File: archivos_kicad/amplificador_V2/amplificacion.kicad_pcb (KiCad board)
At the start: 2 copper layers, 62 x 85.8 mm, 24 parts, among them J1 INPUT_L, J2 OUTPUT_L, J3 ALIMENTACION REJILLA, J4 ALIMENTACION FILAMENTO, J5 INPUT_R, J6 OUTPUT_R

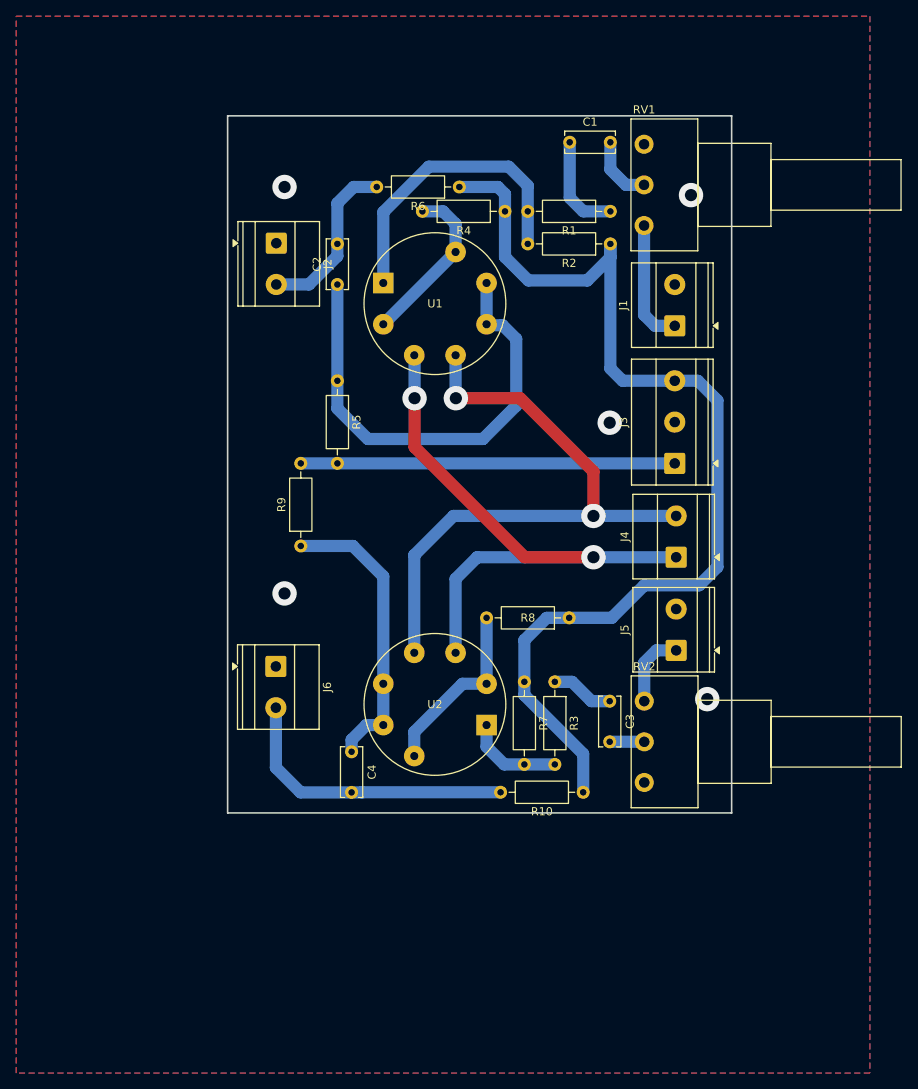
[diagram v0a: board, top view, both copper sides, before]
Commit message: Add files via upload
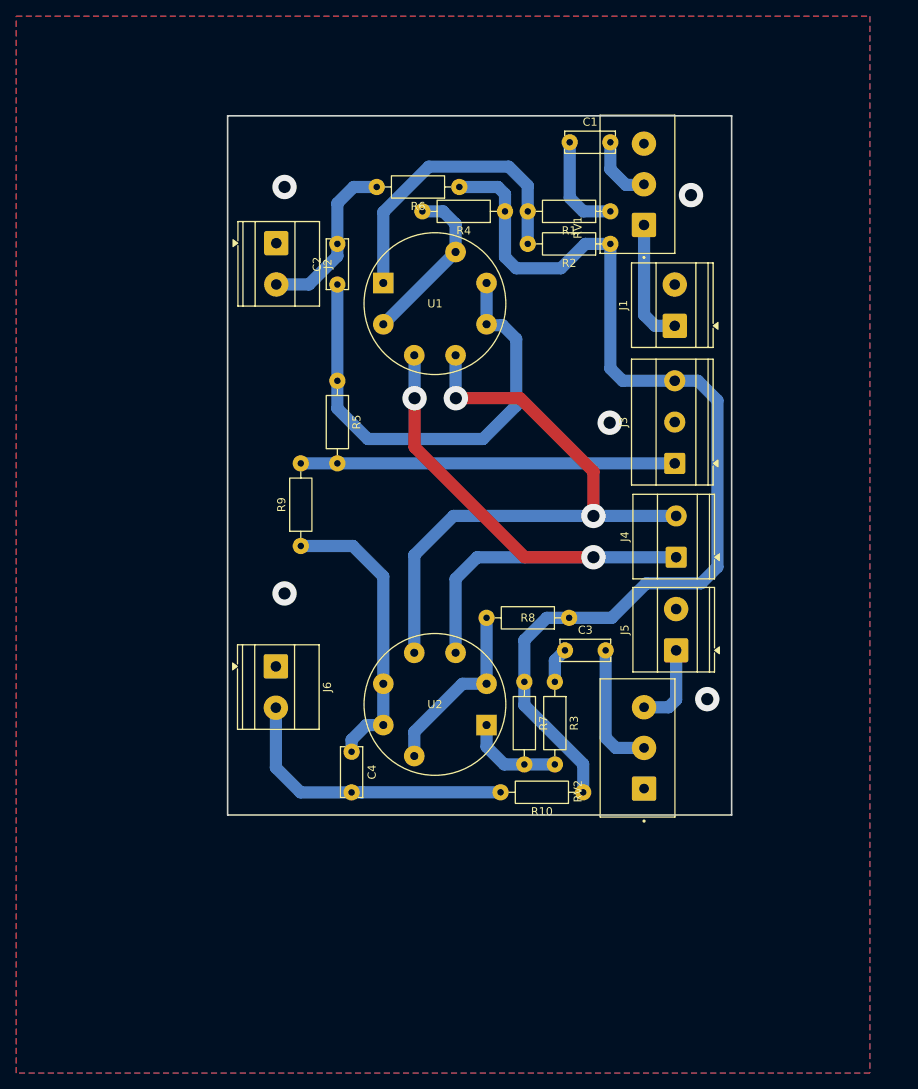
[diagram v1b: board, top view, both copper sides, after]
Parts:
- RV1, RV2: footprint Potentiometer_THT:Potentiometer_Piher_PC-16_Single_Horizontal -> lib_rama:TRIM_WH148-1A-2-18T-L20
- moved C3 8.33 mm to (172.5, 113.0), turned to 0 degrees
- moved RV1 5.07 mm to (182.2, 55.7), turned to 90 degrees
- moved RV2 4.25 mm to (182.2, 125.0), turned to 90 degrees
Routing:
- net Net-(C3-Pad2): track 4.25 -> 16.0 mm
- net Net-(C3-Pad1): track 7.73 -> 4.39 mm
- net -28V: track 130.5 -> 128.3 mm
- net /IN_R: track 9.29 -> 10.4 mm
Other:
- board size 62 x 85.8 mm -> 62 x 86 mm
